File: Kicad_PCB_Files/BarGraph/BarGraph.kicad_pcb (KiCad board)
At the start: 2 copper layers, 30.5 x 98.9 mm, 15 parts, among them J1 USB_B, U1 LED-Bar-Graph, U2 LM3914N

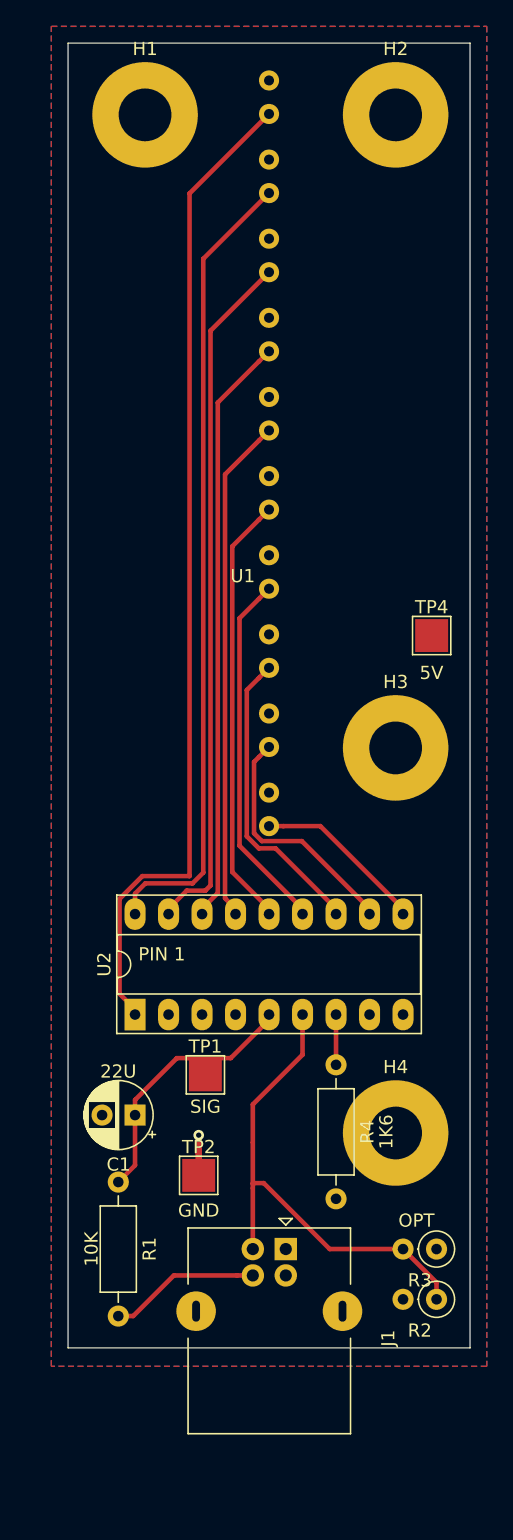
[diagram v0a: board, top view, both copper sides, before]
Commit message: Add files via upload
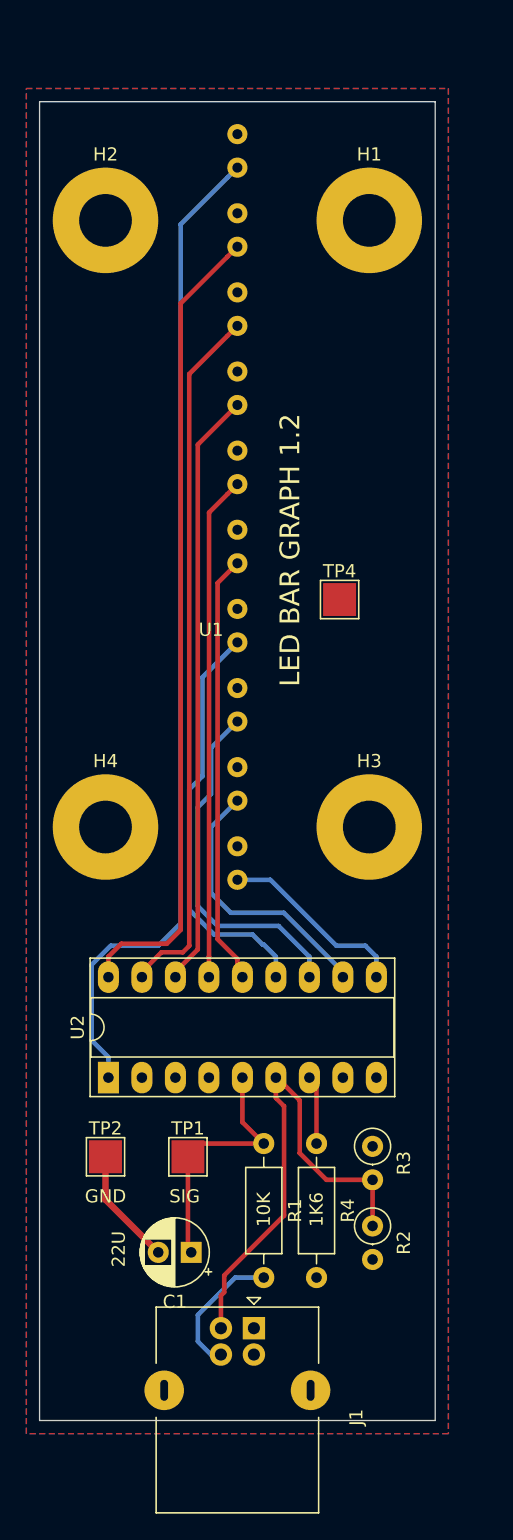
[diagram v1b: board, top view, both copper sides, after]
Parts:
- moved H4 32.0 mm to (140.0, 95.0)
- moved H2 23.4 mm to (140.0, 49.0)
- moved H1 18.8 mm to (160.0, 49.0)
- moved R1 11.4 mm to (152.0, 119.0)
- moved C1 11.2 mm to (146.5, 127.2)
- moved R3 9.18 mm to (160.2, 119.2), turned to 270 degrees
- moved TP4 7.50 mm to (157.8, 77.8)
- moved R2 7.38 mm to (160.2, 125.2), turned to 270 degrees
- moved TP2 7.21 mm to (140.0, 120.0)
- moved J1 6.47 mm to (151.2, 133.0)
- moved TP1 6.35 mm to (146.2, 120.0)
- moved H3 6.32 mm to (160.0, 95.0)
- moved R4 6.15 mm to (156.0, 119.0)
- moved U2 5.19 mm to (140.2, 114.0)
- moved U1 4.72 mm to (150.0, 76.5)
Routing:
- net GND: track 3.05 -> 8.91 mm, vias 1 -> 0
- net Net-(U1-Pad7): track 27.6 -> 31.8 mm
- net Net-(U1-Pad8): track 22.9 -> 26.8 mm
- net Net-(U1-Pad9): track 18.5 -> 20.7 mm
- net Net-(R4-Pad1): track 3.81 -> 5.22 mm
- net Net-(U1-Pad10): track 13.2 -> 14.5 mm
- net Net-(J1-Pad3): track 11.5 -> 10.3 mm
- net Net-(U1-Pad3): track 52.7 -> 53.3 mm
- net Net-(U1-Pad1): track 75.6 -> 76.2 mm
- net Net-(C1-Pad1): track 19.8 -> 19.2 mm
- net Net-(U1-Pad4): track 44.8 -> 45.3 mm
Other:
- board size 30.5 x 98.9 mm -> 30 x 100 mm
- net class Default: clearance 0.2 -> 0.3
- net class Power: clearance 0.2 -> 0.3
- rule trace_clearance: 0.2 -> 0.3
- board text added: "LED BAR GRAPH 1.2"
- board text removed: "5V"
- board text removed: "OPT"
- board text removed: "PIN 1"
